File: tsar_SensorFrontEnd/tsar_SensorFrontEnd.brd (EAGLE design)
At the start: 278.1 x 210.5 mm, 108 parts

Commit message: Reduced board size
fixed missing TVS cap values
modified board layout to reduce size
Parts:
- removed SER: 057-040-1, con-panduit:057-040-1
- added X1: 057-040-1, con-panduit:057-040-1
- C1, C10, C16, C17, C18, C2, C21, C3, C4, C5, C6, C8, C9: value (none) -> 120pF
- C20: value (none) -> 120pf
- C7: value 100n -> 120pF
- moved TP 182.0 mm to (83.2, 18.2), turned to 180 degrees
- moved POE_IN 130.5 mm to (102.2, 81.8)
- moved C19 110.2 mm to (75.3, 70.7)
- moved R26 110.2 mm to (70.0, 70.7)
- moved C15 110.2 mm to (83.7, 66.4)
- moved C23 110.2 mm to (92.6, 55.0)
- moved R30 110.2 mm to (70.0, 67.2)
- moved R33 110.2 mm to (88.0, 50.4)
- moved R34 110.2 mm to (92.6, 49.6)
- moved U$1 110.2 mm to (81.7, 61.8)
- moved U$2 110.2 mm to (81.2, 75.0)
- moved C22 110.2 mm to (92.6, 60.6)
- moved CR1 110.2 mm to (78.1, 65.1)
- moved DFLS160 110.2 mm to (96.4, 65.9)
- moved R21 107.1 mm to (52.5, 74.7)
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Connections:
- removed net N$34: AN.27
- removed net N$35: AN.25
- removed net N$36: AN.23
- net 10: now also AN.23
- net 8: now also AN.27
- net 9: now also AN.25
- net N$10: now also U$1.P$4
- net N$8: now also U$4.P$4
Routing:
- net N$14: track 0.00 -> 83.1 mm
- net N$15: track 0.00 -> 82.2 mm
- net 10: track 4.62 -> 83.2 mm
- net N$16: track 0.00 -> 77.0 mm
- net N$12: track 0.00 -> 75.2 mm
- net +3V3: track 9.22 -> 69.0 mm, vias 0 -> 3
- net 9: track 4.62 -> 64.1 mm
- net 5: track 4.63 -> 62.8 mm
- net 4: track 4.78 -> 56.1 mm
- net 3: track 4.71 -> 54.0 mm
- net 2: track 4.87 -> 49.5 mm
- net 8: track 4.78 -> 44.9 mm
- net 1: track 4.63 -> 43.2 mm
- net GND2: track 0.00 -> 29.8 mm
- net 7: track 4.63 -> 30.9 mm
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- added copper zone on layer 16, net GND
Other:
- board size 278.1 x 210.5 mm -> 195.1 x 91 mm

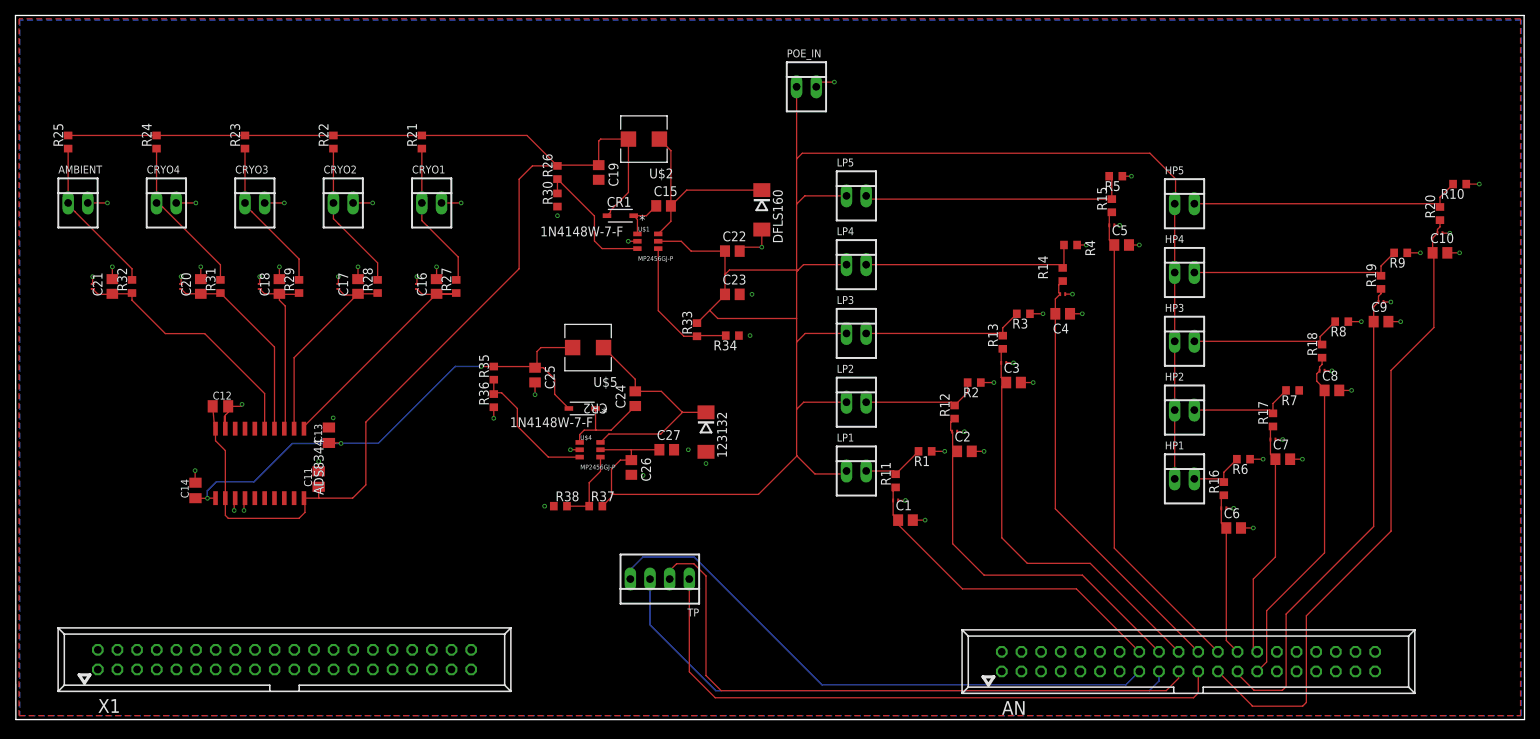
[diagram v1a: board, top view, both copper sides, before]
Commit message: Shrunk Board Layout
Reduced size of board
Replaced 20x2 connectors with marionette library part.
Missing digital pin connections
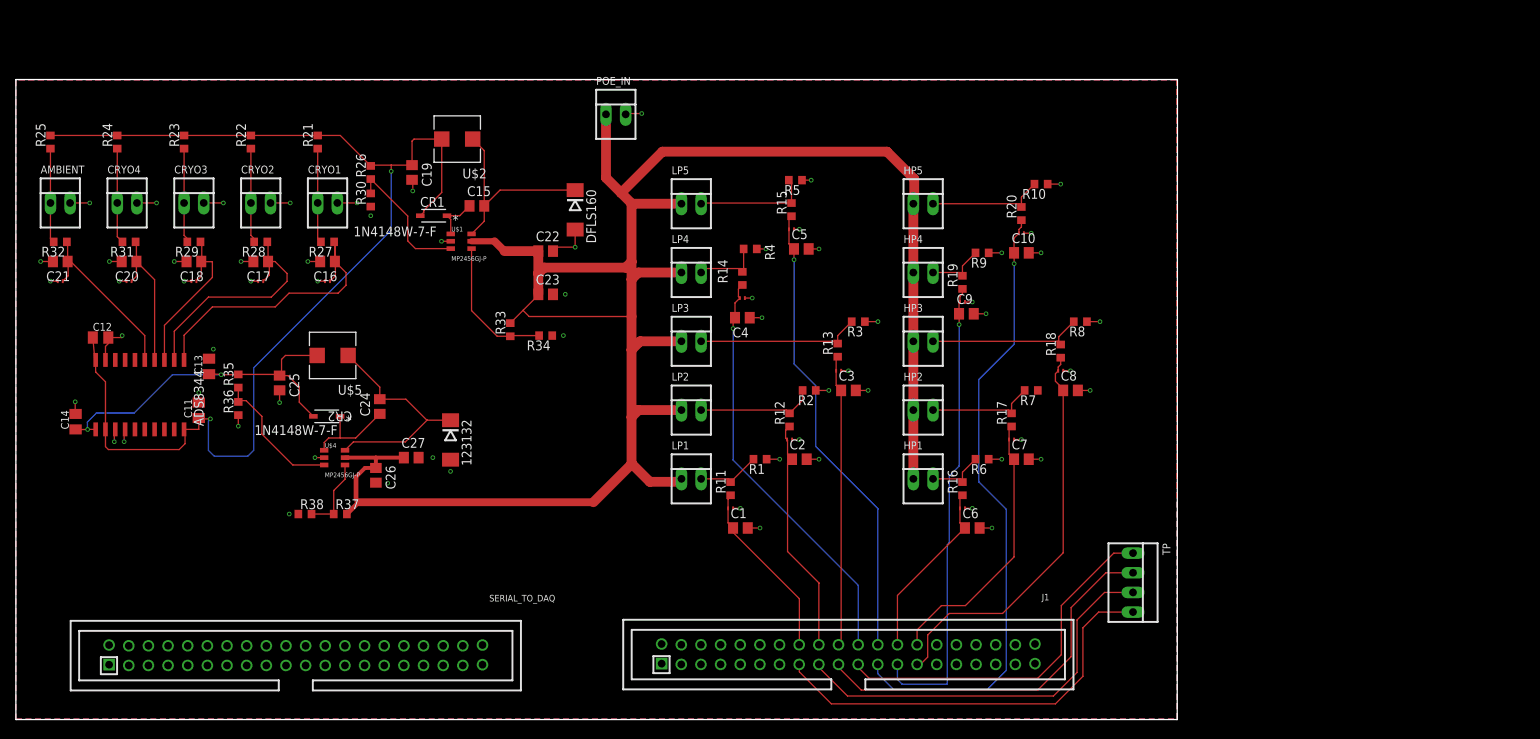
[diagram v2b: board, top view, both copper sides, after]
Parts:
- removed AN, X1: 057-040-1, con-panduit:057-040-1
- added J1, SERIAL_TO_DAQ: IDC_RECEPTACLE_2X20-S9175-ND, marionette:IDC_RECEPTACLES
- moved TP 61.2 mm to (144.4, 17.7), turned to 270 degrees
- moved C10 54.1 mm to (130.0, 60.3)
- moved R10 54.1 mm to (132.5, 69.2)
- moved R19 54.1 mm to (122.4, 56.5)
- moved R20 54.1 mm to (130.0, 65.4)
- moved TVS10 54.1 mm to (130.0, 62.9)
- moved TVS9 54.1 mm to (122.4, 54.0)
- moved R9 54.1 mm to (124.9, 60.3)
- moved C9 53.6 mm to (122.9, 52.5)
- moved C5 41.4 mm to (101.5, 60.8)
- moved R5 41.4 mm to (100.8, 69.7)
- moved C4 41.4 mm to (93.9, 51.9)
- moved R14 41.4 mm to (93.9, 57.0)
- moved R15 41.4 mm to (100.3, 65.9)
- moved R4 41.4 mm to (94.9, 60.8)
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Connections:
- net 1: now also J1.16; no longer AN.16
- net 10: now also J1.23; no longer AN.23
- net 2: now also J1.18; no longer AN.18
- net 3: now also J1.20; no longer AN.20
- net 4: now also J1.22; no longer AN.22
- net 5: now also J1.24; no longer AN.24
- net 6: now also J1.26; no longer AN.26
- net 7: now also J1.28; no longer AN.28
- net 8: now also J1.27; no longer AN.27
- net 9: now also J1.25; no longer AN.25
- net N$12: now also J1.15; no longer AN.15
- net N$14: now also J1.19; no longer AN.19
- net N$15: now also J1.21; no longer AN.21
- net N$16: now also J1.17; no longer AN.17
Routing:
- net N$15: track 82.2 -> 46.9 mm
- net N$14: track 83.1 -> 49.7 mm
- net +5V: track 179.2 -> 153.6 mm, vias 0 -> 2
- net N$16: track 77.0 -> 52.0 mm
- net +3V3: track 69.0 -> 47.4 mm, vias 3 -> 2
- net N$12: track 75.2 -> 54.4 mm
- net N$7: track 28.0 -> 7.64 mm
- net N$46: track 35.5 -> 15.2 mm
- net N$29: track 35.0 -> 14.8 mm
- net 1: track 43.2 -> 23.3 mm
- net N$1: track 28.7 -> 8.80 mm
- net 2: track 49.5 -> 30.8 mm
- net 3: track 54.0 -> 37.7 mm
- net 19: track 33.1 -> 22.8 mm
- net CRYO4: track 20.5 -> 12.3 mm
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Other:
- board size 195.1 x 91 mm -> 150.1 x 82.7 mm
